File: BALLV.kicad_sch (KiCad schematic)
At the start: 3 parts

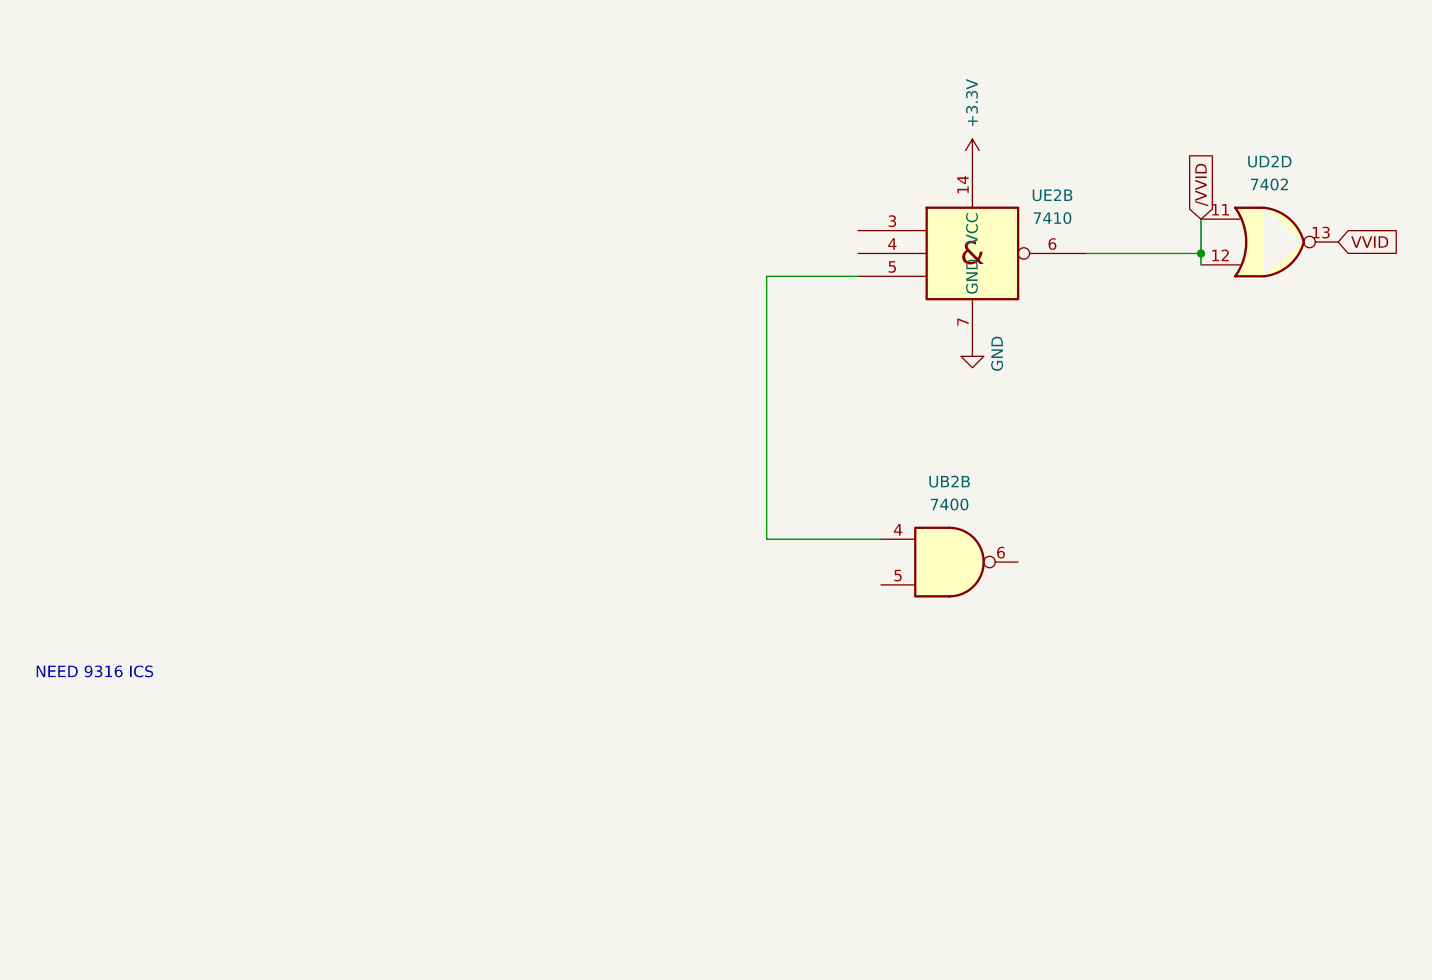
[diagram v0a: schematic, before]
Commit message: R20260922PM
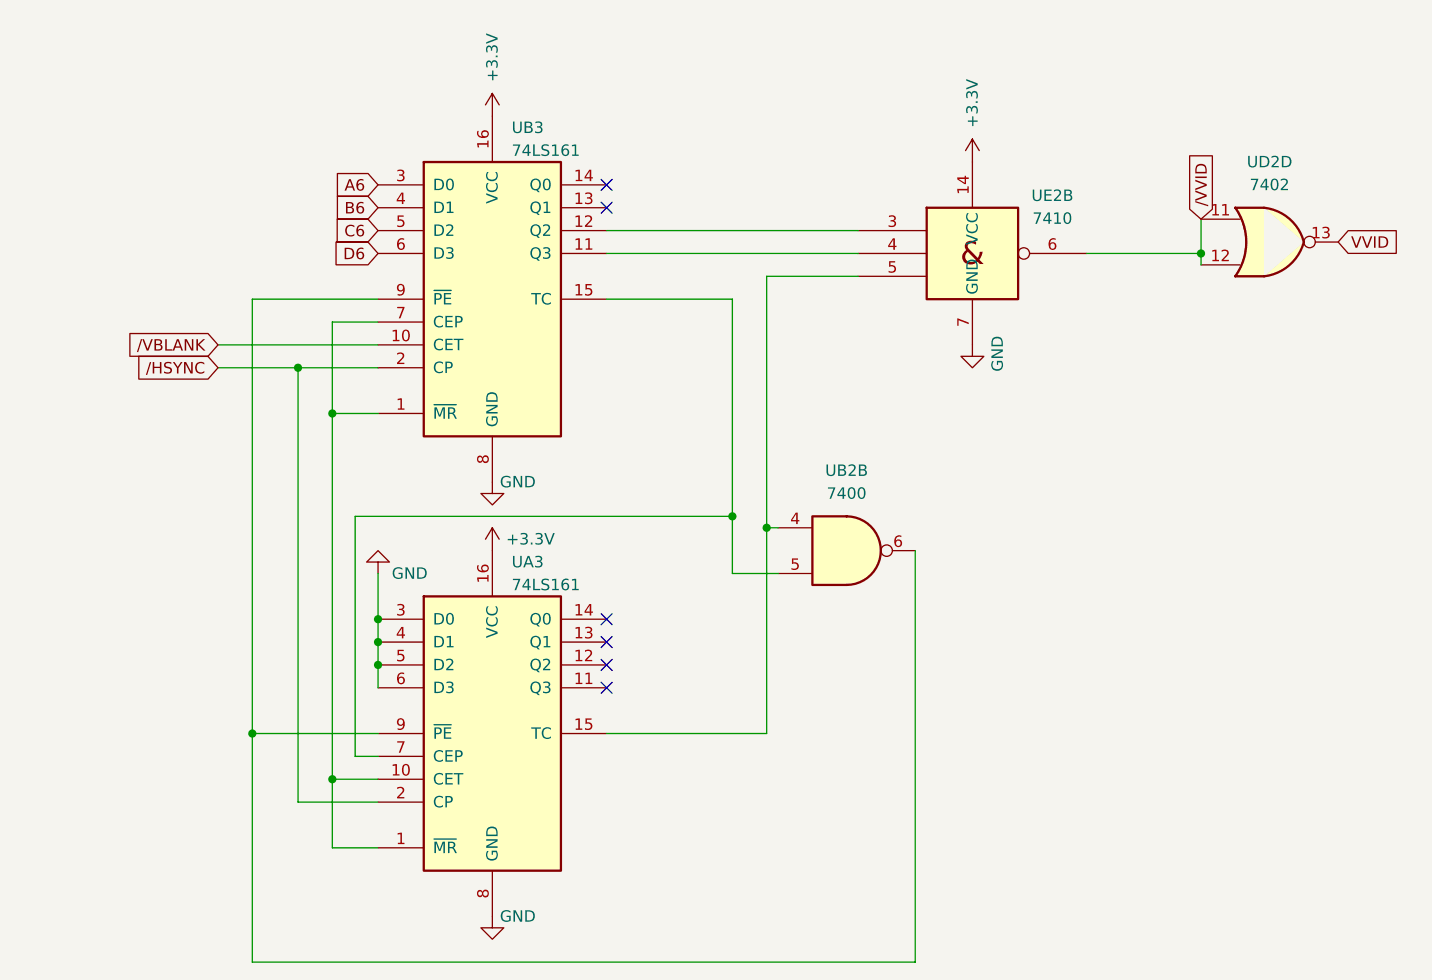
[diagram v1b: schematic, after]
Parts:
- added UA3, UB3: 74LS161, pong:pong_DIP-16_W7.62mm_Socket_LongPads, symbol 74xx:74LS161
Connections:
- net +3.3V: now also UA3.16 (VCC), UB3.16 (VCC)
- net GND: now also UA3.3 (D0), UA3.4 (D1), UA3.5 (D2), UA3.6 (D3), UA3.8 (GND), UB3.8 (GND)
- net at UB2.4, UE2.5: now also UA3.15 (TC)
- net at UB2.5: now also UA3.7 (CEP), UB3.15 (TC)
- net at UB2.6: now also UA3.9 (~{PE}), UB3.9 (~{PE})
- net at UE2.3: now also UB3.12 (Q2)
- net at UE2.4: now also UB3.11 (Q3)
- new net: UA3.1 (~{MR}), UA3.10 (CET), UB3.1 (~{MR}), UB3.7 (CEP)
- new net A6: UB3.3 (D0)
- new net B6: UB3.4 (D1)
- new net C6: UB3.5 (D2)
- new net D6: UB3.6 (D3)
- new net /HSYNC: UA3.2 (CP), UB3.2 (CP)
- new net /VBLANK: UB3.10 (CET)
- no-connect marks 0 -> 6
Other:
- note removed: "NEED 9316 ICS"
- moved on the sheet: UB2B
